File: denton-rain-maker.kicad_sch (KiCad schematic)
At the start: 68 parts, among them J1 Conn_01x06, J2 MOV, J3 SEED C3, Q4 BT136S-800E, Q5 BT136S-800E, Q6 BT136S-800E, Q7 BT136S-800E, U1 LMR38020FSDDAR, U2 TLV1117-33, U4 MOC3063M, U6 MOC3063M, U7 MOC3063M, U8 MOC3063M

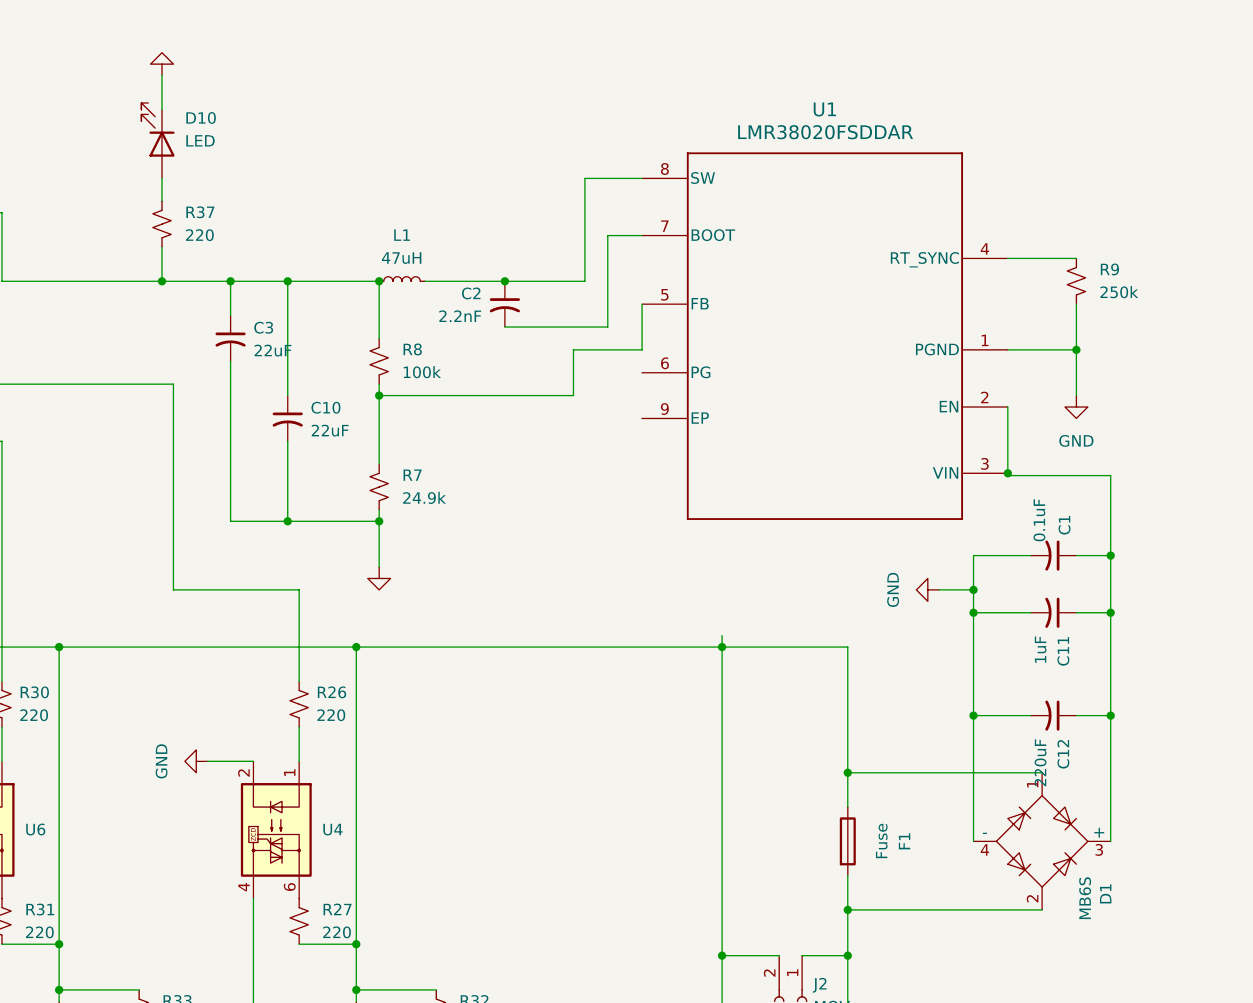
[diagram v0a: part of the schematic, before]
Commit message: new pwr supply
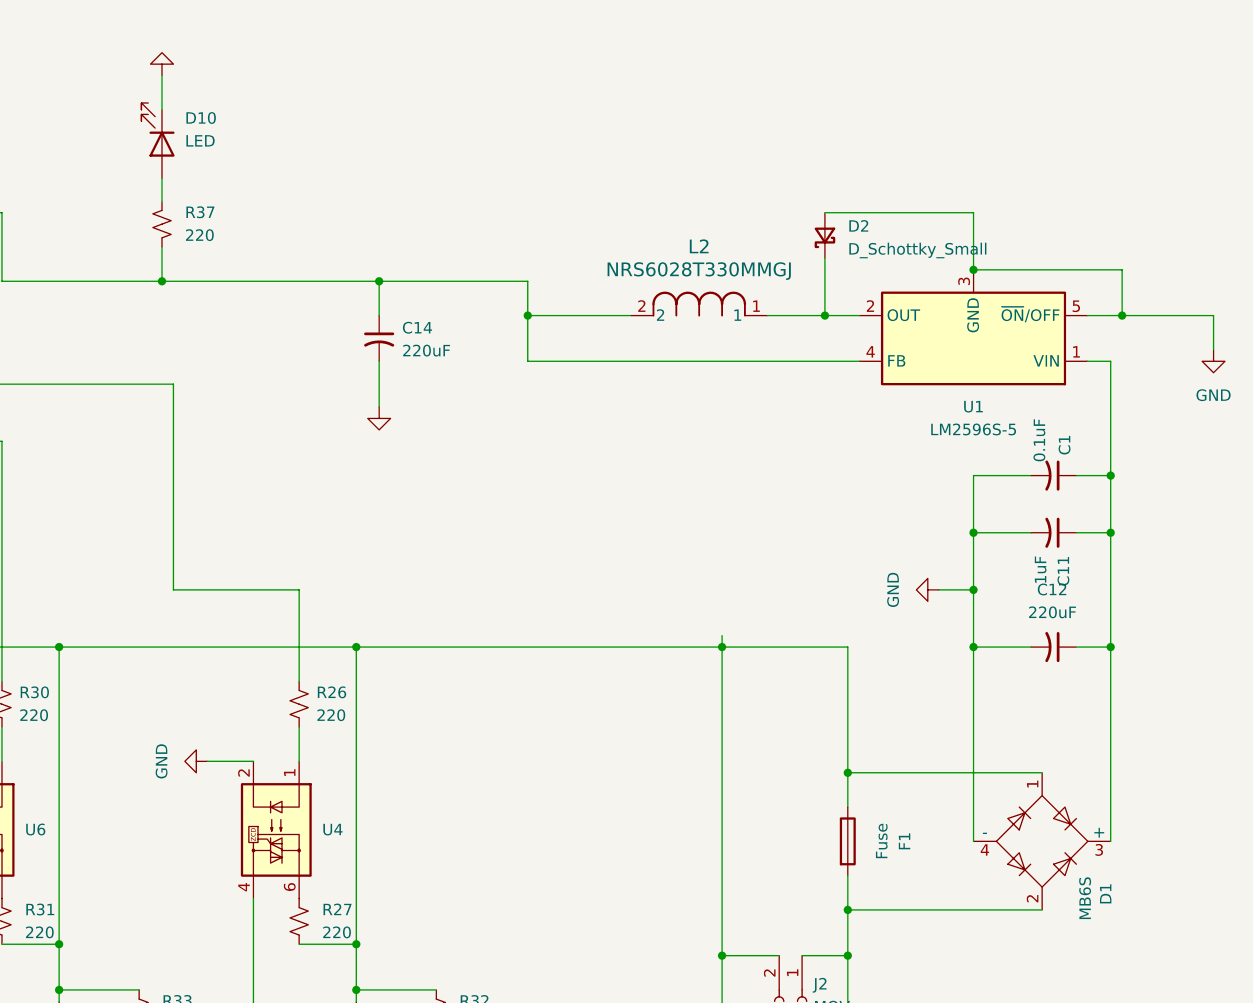
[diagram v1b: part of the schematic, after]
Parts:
- removed C10, C3: 22uF, Capacitor_SMD:C_1206_3216Metric_Pad1.33x1.80mm_HandSolder, symbol Device:C_Small_US
- removed C2: 2.2nF, Capacitor_SMD:C_1206_3216Metric_Pad1.33x1.80mm_HandSolder, symbol Device:C_Small_US
- removed L1: 47uH, Inductor_SMD:L_Bourns_SRN6045TA, symbol Device:L_Small
- removed R7: 24.9k, Resistor_SMD:R_1206_3216Metric_Pad1.30x1.75mm_HandSolder, symbol Device:R_Small_US
- removed R8: 100k, Resistor_SMD:R_1206_3216Metric_Pad1.30x1.75mm_HandSolder, symbol Device:R_Small_US
- removed R9: 250k, Resistor_SMD:R_1206_3216Metric_Pad1.30x1.75mm_HandSolder, symbol Device:R_Small_US
- removed U1: LMR38020FSDDAR, footprints:DDA0008E-IPC_C, symbol 2026-06-20_16-52-41:LMR38020FSDDAR
- added C14: 220uF, Capacitor_THT:CP_Radial_D10.0mm_P5.00mm, symbol Device:C_Small_US
- added D2: D_Schottky_Small, Diode_SMD:D_MicroSMP_LargeCathode, symbol Device:D_Schottky_Small
- added L2: NRS6028T330MMGJ, inductor:IND_TAIYO_NRS6028_TAY, symbol 2026-06-23_19-00-12:NRS6028T330MMGJ
- added U1: LM2596S-5, Package_TO_SOT_SMD:TO-263-5_TabPin3, symbol Regulator_Switching:LM2596S-5
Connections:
- net GND: now also C14.2, D2.2 (A), U1.3 (GND), U1.5 (~{ON}/OFF)
- net at C9.1, R37.2, U2.3 (VI): now also C14.1, L2.2, U1.4 (FB)
- net at C1.1, C11.1, C12.1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: now also U1.1 (VIN)
- new net: D2.1 (K), L2.1, U1.2 (OUT)
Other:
- moved on the sheet: C1, C11, C12
